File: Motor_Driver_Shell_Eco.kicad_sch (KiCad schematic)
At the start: 0 parts

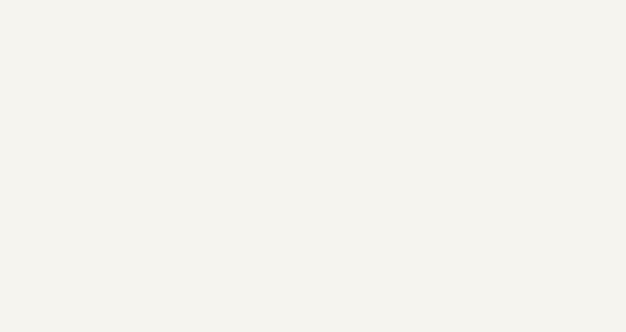
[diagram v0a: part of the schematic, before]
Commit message: bit artık
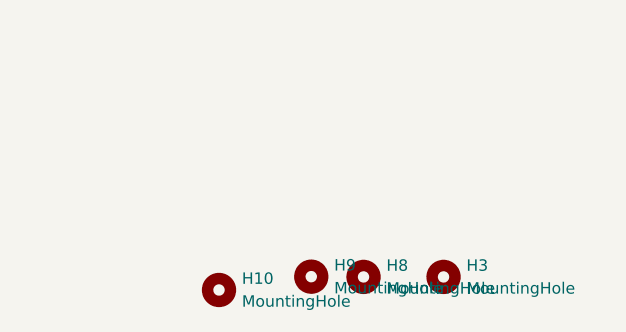
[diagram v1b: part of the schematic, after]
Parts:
- added H10, H3, H8, H9: MountingHole, MountingHole:MountingHole_2.2mm_M2, symbol Mechanical:MountingHole
